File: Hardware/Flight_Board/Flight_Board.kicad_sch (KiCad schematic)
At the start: 0 parts

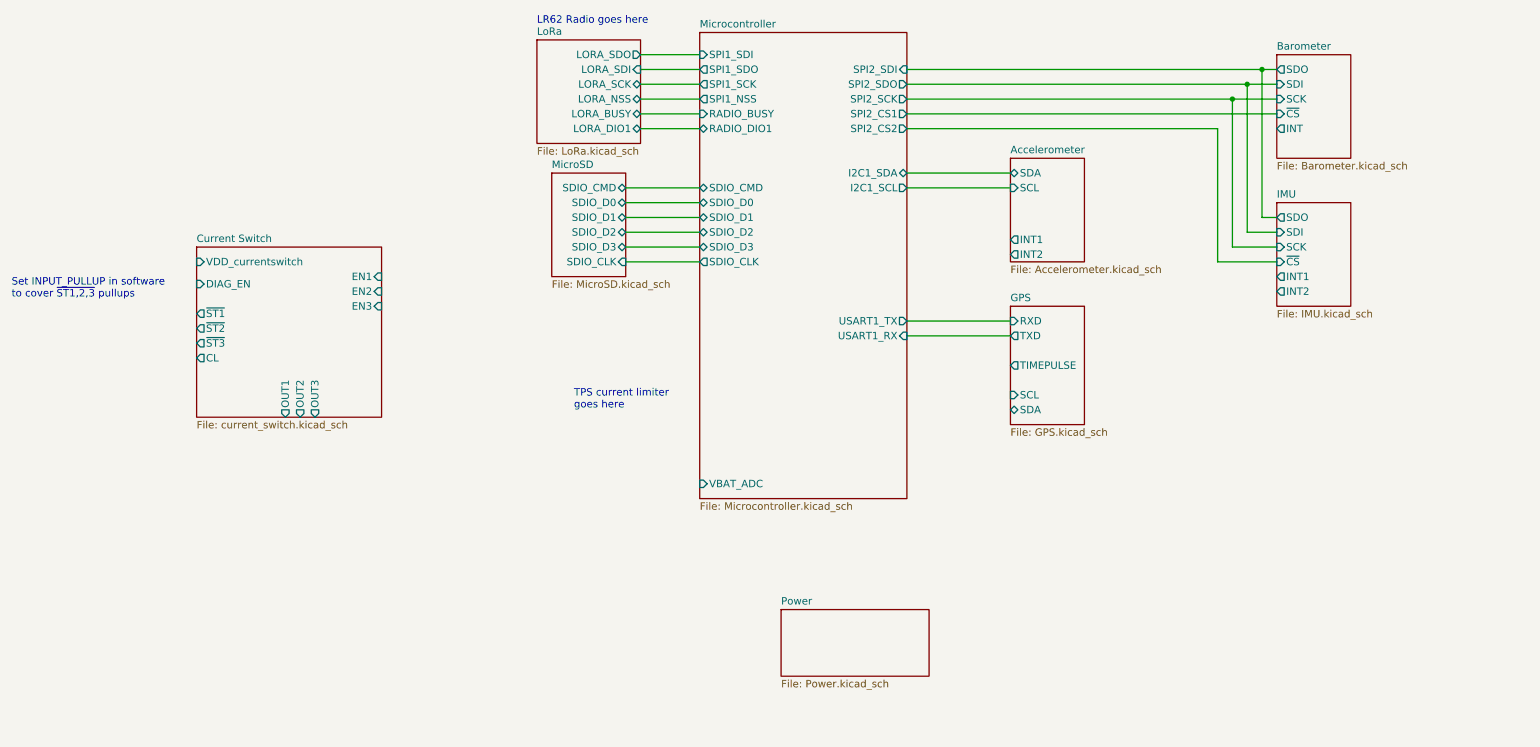
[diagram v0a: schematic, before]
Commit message: clean up and finalize initial design
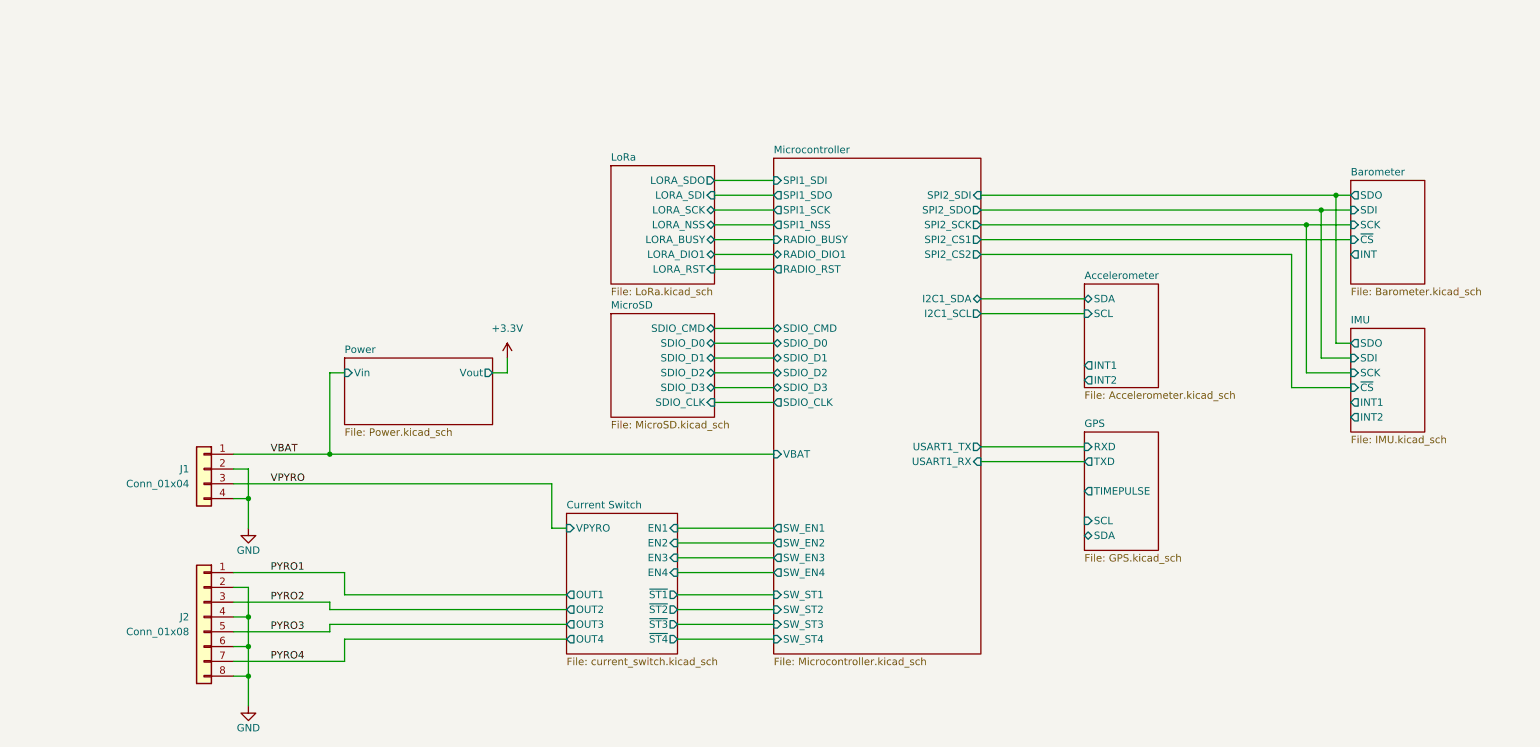
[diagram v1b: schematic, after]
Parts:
- added J1: Conn_01x04, symbol Connector_Generic:Conn_01x04
- added J2: Conn_01x08, symbol Connector_Generic:Conn_01x08
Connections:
- new net GND: J1.2 (Pin_2), J1.4 (Pin_4), J2.2 (Pin_2), J2.4 (Pin_4), J2.6 (Pin_6), J2.8 (Pin_8)
- new net PYRO1: J2.1 (Pin_1)
- new net PYRO2: J2.3 (Pin_3)
- new net PYRO3: J2.5 (Pin_5)
- new net PYRO4: J2.7 (Pin_7)
- new net VBAT: J1.1 (Pin_1)
- new net VPYRO: J1.3 (Pin_3)
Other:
- sheet Current Switch ports: added EN4, OUT4, VPYRO, ~{ST4}; removed CL, DIAG_EN, VDD_currentswitch
- sheet LoRa ports: added LORA_RST; removed none
- sheet Microcontroller ports: added RADIO_RST, SW_EN1, SW_EN2, SW_EN3, SW_EN4, SW_ST1, SW_ST2, SW_ST3, SW_ST4, VBAT; removed VBAT_ADC
- sheet Power ports: added Vin, Vout; removed none
- note removed: "LR62 Radio goes here"
- note removed: "Set INPUT_PULLUP in software to cover ~{ST1,2,3} pullups"
- note removed: "TPS current limiter goes here"
